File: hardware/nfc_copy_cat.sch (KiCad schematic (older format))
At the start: 36 parts, among them J1 USB_B_Micro, J2 Battery, J3 SWD, J4 NFC Module V3, J5 Conn_01x02, J6 Adafruit NFC 1.0, SW1 RST, SW2 Magspoof, SW3 NFC, U1 AP2112K-3.3TRG1, U2 MCP73831-2-OT, U3 TC4424, U4 ATSAMD21E18A, U5 W25Q16JVSS

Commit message: netlist
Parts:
- C3: footprint (none) -> Capacitor_SMD:C_0805_2012Metric_Pad1.15x1.40mm_HandSolder
- J3: footprint (none) -> Connector_PinHeader_2.54mm:PinHeader_1x04_P2.54mm_Vertical
- R7: footprint (none) -> Resistor_SMD:R_0805_2012Metric_Pad1.15x1.40mm_HandSolder
- U1: symbol electroniccats:AP2112K-3.3TRG1 -> nfc_copy_cat-rescue:AP2112K-3.3TRG1-electroniccats
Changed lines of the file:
@@
 $EndComp
 $Comp
-L electroniccats:AP2112K-3.3TRG1 U1
+L nfc_copy_cat-rescue:AP2112K-3.3TRG1-electroniccats U1
 U 1 1 5D11FC1B
 P 2325 2825
@@
 F 0 "J3" V 4607 3434 50  0000 L CNN
 F 1 "SWD" V 4698 3434 50  0000 L CNN
-F 2 "" H 4545 3290 50  0001 C CNN
+F 2 "Connector_PinHeader_2.54mm:PinHeader_1x04_P2.54mm_Vertical" H 4545 3290 50  0001 C CNN
 F 3 "~" H 4545 3290 50  0001 C CNN
 	1    4545 3290
@@
 F 0 "C3" H 6220 5891 50  0000 L CNN
 F 1 "0.1uF" H 6220 5800 50  0000 L CNN
-F 2 "" H 6143 5695 50  0001 C CNN
+F 2 "Capacitor_SMD:C_0805_2012Metric_Pad1.15x1.40mm_HandSolder" H 6143 5695 50  0001 C CNN
 F 3 "~" H 6105 5845 50  0001 C CNN
 	1    6105 5845
@@
 F 0 "R7" H 4155 5626 50  0000 L CNN
 F 1 "100K" H 4125 5550 50  0000 L CNN
-F 2 "" V 4015 5580 50  0001 C CNN
+F 2 "Resistor_SMD:R_0805_2012Metric_Pad1.15x1.40mm_HandSolder" V 4015 5580 50  0001 C CNN
 F 3 "~" H 4085 5580 50  0001 C CNN
 	1    4085 5580

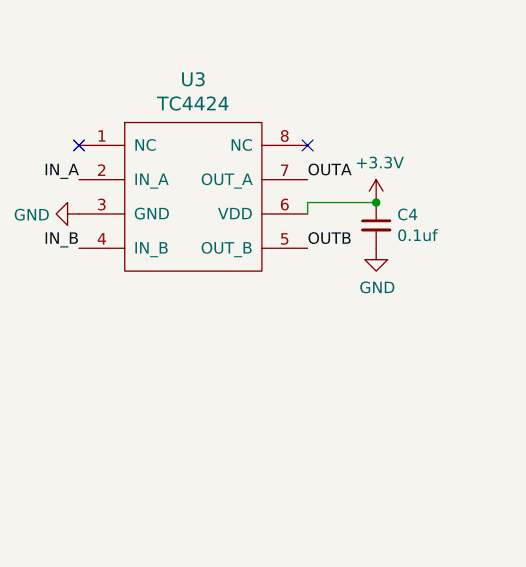
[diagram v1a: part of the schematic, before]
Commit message: chance c4 eschema
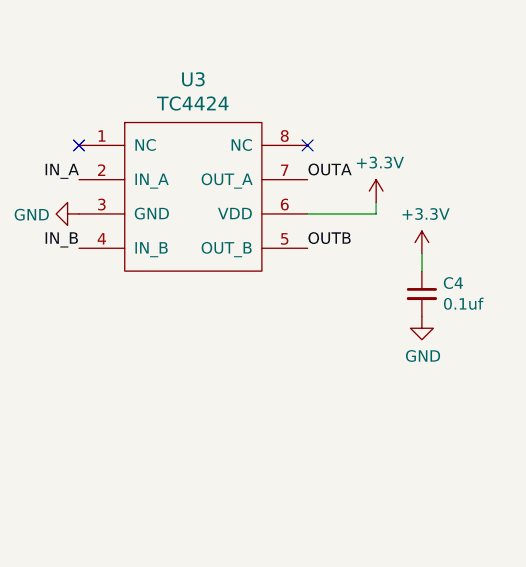
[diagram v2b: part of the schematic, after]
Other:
- moved on the sheet: C4
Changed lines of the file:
@@
 12(MISO)
-$Comp
-L Device:C_Small C4
-U 1 1 5D11FCB0
-P 10620 2470
-F 0 "C4" H 10712 2516 50  0000 L CNN
-F 1 "0.1uf" H 10712 2425 50  0000 L CNN
-F 2 "Capacitor_SMD:C_0805_2012Metric_Pad1.15x1.40mm_HandSolder" H 10620 2470 50  0001 C CNN
-F 3 "~" H 10620 2470 50  0001 C CNN
-	1    10620 2470
-	1    0    0    -1
-$EndComp
 $Comp
 L Connector_Generic:Conn_01x02 J5
@@
 Text Label 9320 2270 2    50   ~ 0
 IN_A
-$Comp
-L power:+3.3V #PWR019
-U 1 1 5D10F76C
-P 10620 2370
-F 0 "#PWR019" H 10620 2220 50  0001 C CNN
-F 1 "+3.3V" H 10635 2543 50  0000 C CNN
-F 2 "" H 10620 2370 50  0001 C CNN
-F 3 "" H 10620 2370 50  0001 C CNN
-	1    10620 2370
-	1    0    0    -1
-$EndComp
-$Comp
-L nfc_copy_cat-rescue:GND-MagSpoofTC-cache #PWR020
-U 1 1 5D11661F
-P 10620 2570
-F 0 "#PWR020" H 10620 2320 50  0001 C CNN
-F 1 "GND" H 10625 2397 50  0000 C CNN
-F 2 "" H 10620 2570 50  0000 C CNN
-F 3 "" H 10620 2570 50  0000 C CNN
-	1    10620 2570
-	1    0    0    -1
-$EndComp
 $Comp
 L Device:Polyfuse F1
@@
 	1    0    0    -1
 $EndComp
-Connection ~ 10620 2370
-Wire Wire Line
-	10320 2370 10620 2370
-Wire Wire Line
-	10320 2420 10320 2370
 $Comp
 L nfc_copy_cat-rescue:GND-MagSpoofTC-cache #PWR016
@@
 Text Label 9320 2570 2    50   ~ 0
 IN_B
-Text Label 10320 2570 0    50   ~ 0
-OUTB
 $Comp
 L nfc_copy_cat-rescue:TC4424-MagSpoofTC-cache U3
@@
 	1700 3410 2310 3410
 NoConn ~ 2780 5960
+$Comp
+L power:+3.3V #PWR?
+U 1 1 5E3E4F66
+P 10820 2595
+F 0 "#PWR?" H 10820 2445 50  0001 C CNN
+F 1 "+3.3V" H 10835 2768 50  0000 C CNN
+F 2 "" H 10820 2595 50  0001 C CNN
+F 3 "" H 10820 2595 50  0001 C CNN
+	1    10820 2595
+	1    0    0    -1
+$EndComp
+Text Label 10320 2570 0    50   ~ 0
+OUTB
+$Comp
+L nfc_copy_cat-rescue:GND-MagSpoofTC-cache #PWR020
+U 1 1 5D11661F
+P 10820 2870
+F 0 "#PWR020" H 10820 2620 50  0001 C CNN
+F 1 "GND" H 10825 2697 50  0000 C CNN
+F 2 "" H 10820 2870 50  0000 C CNN
+F 3 "" H 10820 2870 50  0000 C CNN
+	1    10820 2870
+	1    0    0    -1
+$EndComp
+$Comp
+L power:+3.3V #PWR019
+U 1 1 5D10F76C
+P 10620 2370
+F 0 "#PWR019" H 10620 2220 50  0001 C CNN
+F 1 "+3.3V" H 10635 2543 50  0000 C CNN
+F 2 "" H 10620 2370 50  0001 C CNN
+F 3 "" H 10620 2370 50  0001 C CNN
+	1    10620 2370
+	1    0    0    -1
+$EndComp
+$Comp
+L Device:C_Small C4
+U 1 1 5D11FCB0
+P 10820 2770
+F 0 "C4" H 10912 2816 50  0000 L CNN
+F 1 "0.1uf" H 10912 2725 50  0000 L CNN
+F 2 "Capacitor_SMD:C_0805_2012Metric_Pad1.15x1.40mm_HandSolder" H 10820 2770 50  0001 C CNN
+F 3 "~" H 10820 2770 50  0001 C CNN
+	1    10820 2770
+	1    0    0    -1
+$EndComp
+Wire Wire Line
+	10820 2670 10820 2595
+Wire Wire Line
+	10320 2420 10620 2420
+Wire Wire Line
+	10620 2420 10620 2370
 $EndSCHEMATC
